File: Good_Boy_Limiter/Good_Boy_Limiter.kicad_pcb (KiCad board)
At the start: 2 copper layers, 105.4 x 86.5 mm, 106 parts, among them CN1 XT30PW-M, CN2 XT30PW-M, J2 Extra General Pins, Q1 STB15810, Q2 AO3422, Q4 AO3400A, SW3 RESET1, SW4 BOOT1, U1 ESP32-S3-WROOM-1, U10 B3B-XH-A, U11 B3B-XH-A, U12 B3B-XH-A, U2 1-178136-3, U3 LM5069MM-2/NOPB, U4 USBLC6-2SC6, U5 SY8120B, U7 LM5013DDAR, U8 B3B-XH-A

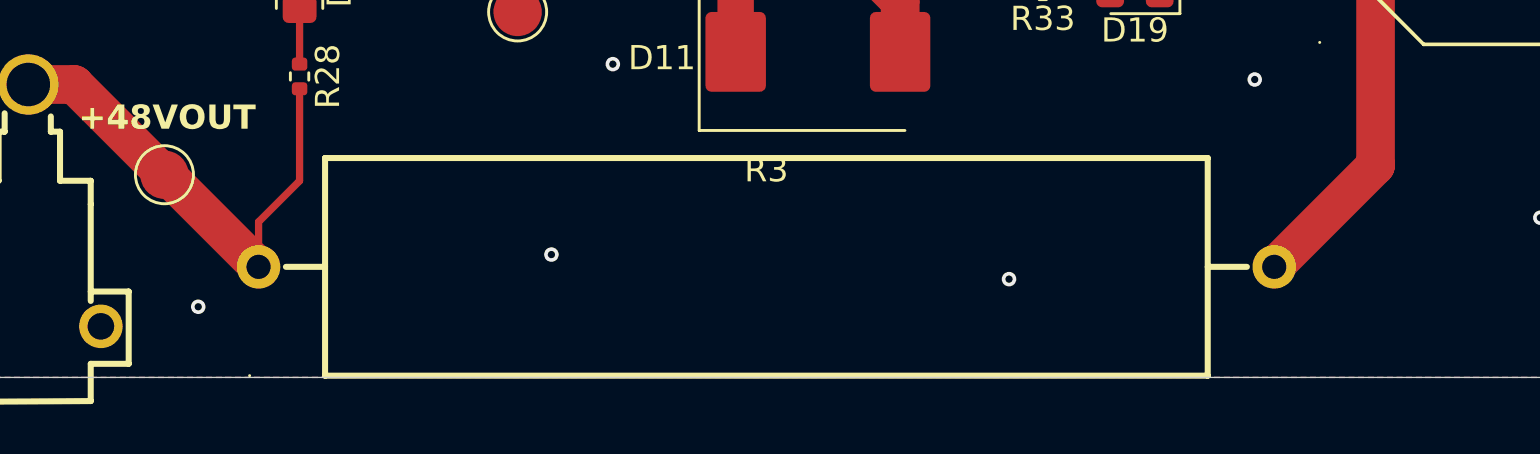
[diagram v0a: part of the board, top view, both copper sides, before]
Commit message: Added pictures and title page
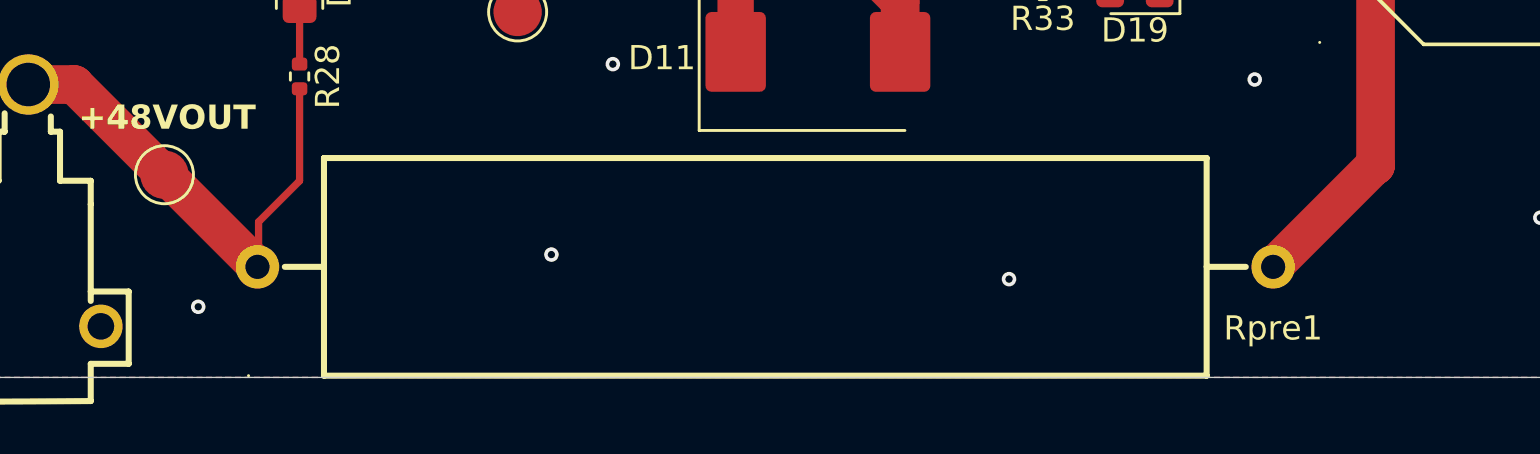
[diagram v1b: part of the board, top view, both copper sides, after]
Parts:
- removed R3: 50ohm, easyeda2kicad:RES-TH_BD9.0-L36.5-P40.50-D0.8
- added Rpre1: 50ohm, easyeda2kicad:RES-TH_BD9.0-L36.5-P40.50-D0.8, F.Cu at (186.6, 114.3)

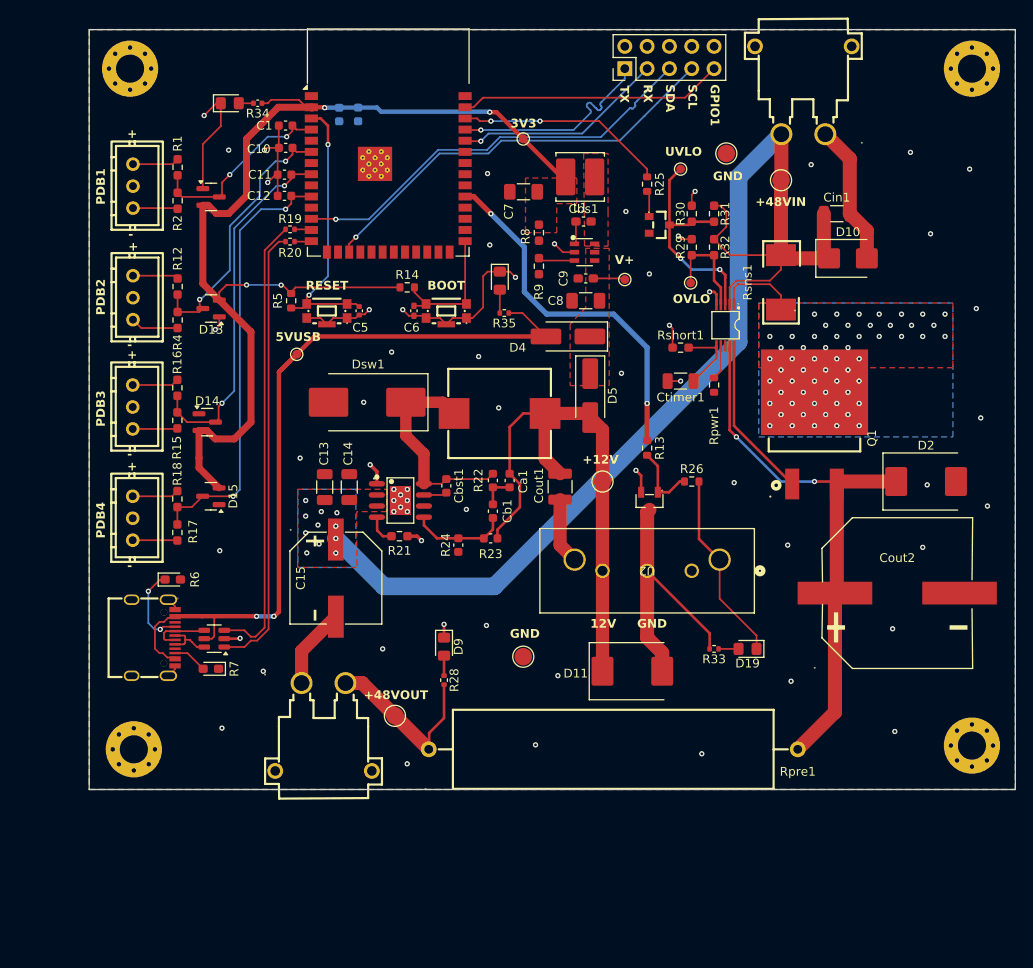
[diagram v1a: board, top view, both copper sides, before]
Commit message: Documentation update
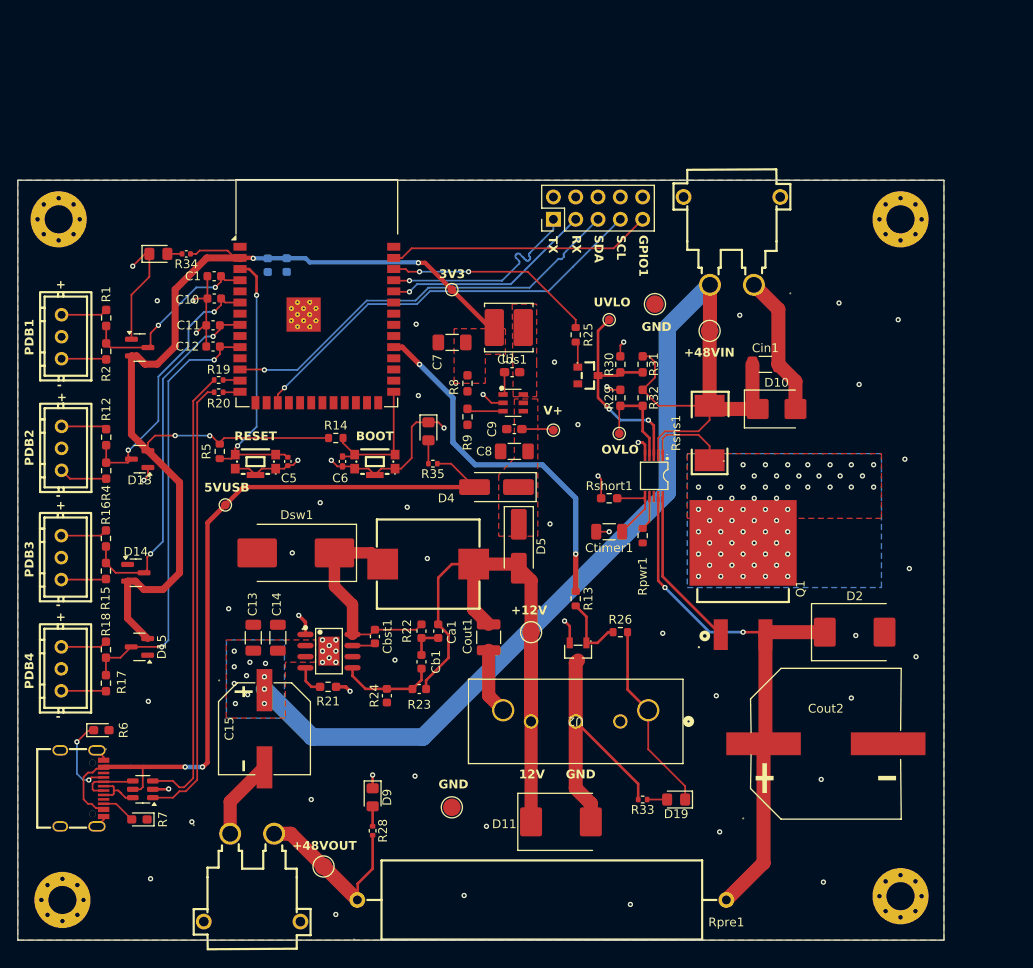
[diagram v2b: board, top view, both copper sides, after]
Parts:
- moved C5 19.0 mm to (149.6, 81.5)
- moved L3 19.0 mm to (165.6, 93.2)
- moved Q1 19.0 mm to (201.4, 96.0)
- moved R26 19.0 mm to (187.5, 101.0)
- moved R4 19.0 mm to (128.9, 82.6)
- moved Rpwr1 19.0 mm to (190.0, 90.0)
- moved TP8 19.0 mm to (153.7, 127.6)
- moved C3 19.0 mm to (147.3, 59.2)
- moved CN2 19.0 mm to (200.2, 56.4)
- moved J2 19.0 mm to (179.8, 54.0)
- moved R12 19.0 mm to (128.9, 78.8)
- moved R19 19.0 mm to (141.7, 72.3)
- moved R29 19.0 mm to (187.5, 74.3)
- moved R32 19.0 mm to (190.0, 74.3)
- moved R8 19.0 mm to (170.1, 72.6)
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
